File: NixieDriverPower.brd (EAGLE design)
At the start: 43.2 x 34.9 mm, 18 parts, among them IC1 MC34063AD, T1 MJD31

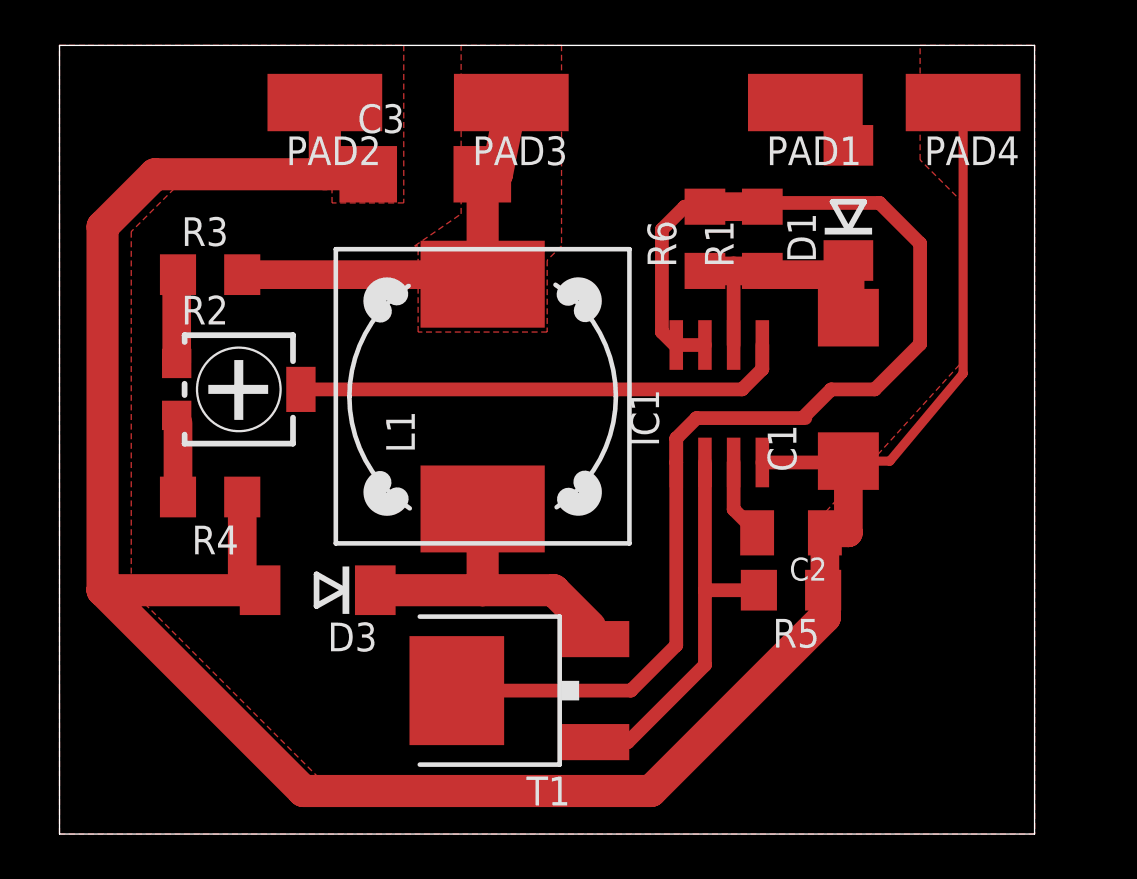
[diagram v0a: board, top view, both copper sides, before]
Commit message: Commit of the current version
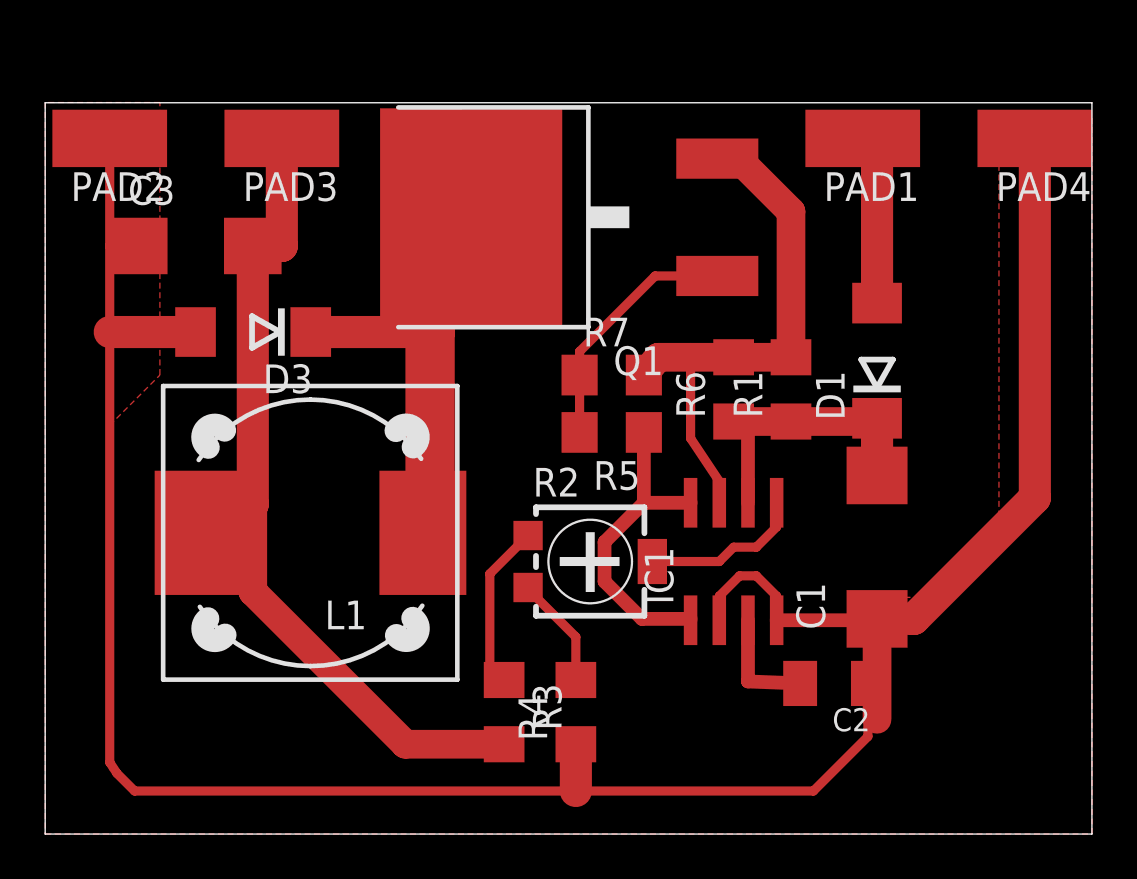
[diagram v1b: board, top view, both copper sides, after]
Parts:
- removed T1: MJD31, transistor:DPAK
- added Q1: IRF4905D2PAK, own-collection:D2PAK
- added R7: 360, rcl-2:R1206
- R5: value 1.5k -> 200
- moved R3 23.3 mm to (20.3, 5.40), turned to 270 degrees
- moved R4 18.8 mm to (23.5, 5.40), turned to 90 degrees
- moved R2 17.3 mm to (24.1, 12.1)
- moved D3 11.8 mm to (9.21, 22.2)
- moved C3 10.6 mm to (6.67, 26.0)
- moved R5 10.6 mm to (25.1, 17.8)
- moved PAD3 10.3 mm to (10.5, 30.8)
- moved L1 9.72 mm to (11.7, 13.3), turned to 180 degrees
- moved PAD2 9.66 mm to (2.86, 30.8)
- moved D1 7.10 mm to (36.8, 21.0)
- moved C1 7.10 mm to (36.8, 12.7)
- moved IC1 7.01 mm to (30.5, 12.1)
- moved C2 6.93 mm to (34.9, 6.67)
- moved R1 6.79 mm to (33.0, 19.7)
- moved R6 6.79 mm to (30.5, 19.7)
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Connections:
- removed net N$3: IC1.1, IC1.7, IC1.8, R1.2, R6.2, T1.4
- new net N$10: IC1.1, IC1.8, R5.1
- new net N$5: IC1.7, Q1.3, R1.2, R6.2, R7.2
- net GND: now also IC1.2; no longer R5.1
- net N$1: now also Q1.4; no longer T1.3
- net N$4: now also Q1.1, R7.1; no longer IC1.2, T1.1
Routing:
- net N$3: track 56.3 -> 0.00 mm
- net N$5: track 0.00 -> 25.0 mm
- net N$6: track 19.5 -> 39.0 mm
- net N$7: track 21.9 -> 7.21 mm
- net N$10: track 0.00 -> 13.9 mm
- net N$1: track 14.6 -> 21.8 mm
- net N$4: track 17.6 -> 11.1 mm
- net N$12: track 3.80 -> 7.68 mm
- net N$9: track 3.94 -> 7.73 mm
- net N$2: track 3.55 -> 5.02 mm
- net N$8: track 3.62 -> 4.97 mm
- net GND: track 114.6 -> 113.4 mm
- removed copper zone on layer 1, net N$6
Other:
- board size 43.2 x 34.9 mm -> 46.3 x 32.4 mm
